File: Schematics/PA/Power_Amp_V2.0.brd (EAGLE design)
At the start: 50.5 x 78.1 mm, 109 parts, among them J1 4_PIN_AMPCONN, J10 OSTVN03A150, J11 OSTVN03A150, J12 OSTVN03A150, J13 OSTVN03A150, J14 OSTVN03A150, J2 1984633, J3 2TERMINAL_SPEAKER, J4 2TERMINAL_SPEAKER, J5 2TERMINAL_SPEAKER, J6 OSTVN03A150, J7 OSTVN03A150, J8 OSTVN03A150, J9 OSTVN03A150, U1 LME49830, U2 LME49830, U3 LME49830

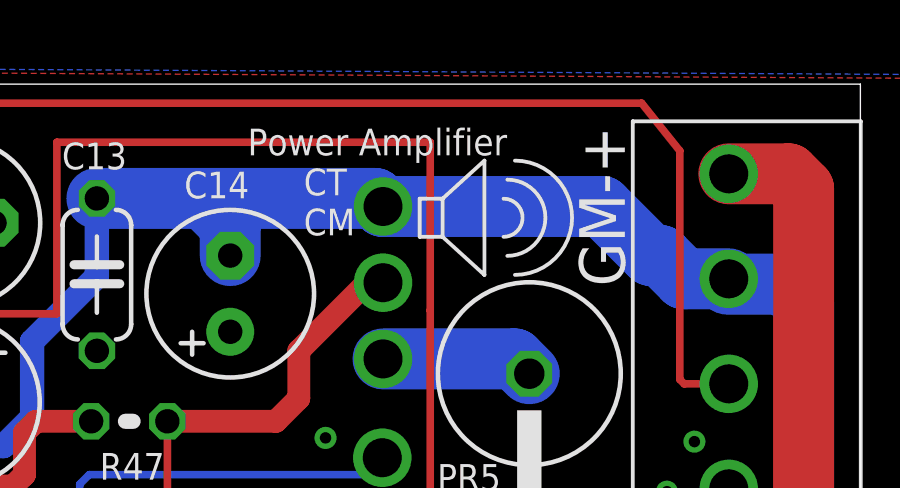
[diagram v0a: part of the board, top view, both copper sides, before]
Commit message: small changes to logo
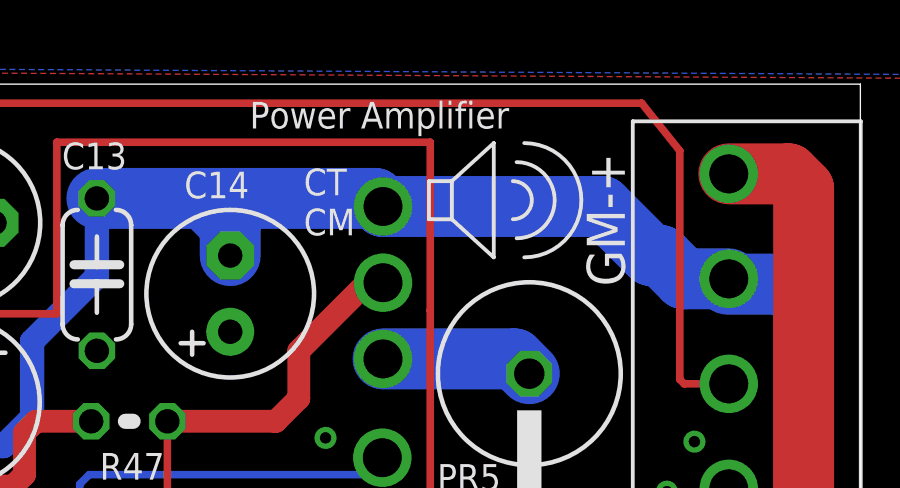
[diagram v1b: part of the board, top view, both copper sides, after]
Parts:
- moved U$48 0.66 mm to (35.6, 74.2)
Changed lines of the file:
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@@
 <grid distance="0.003125" unitdist="mic" unit="inch" style="lines" multiple="1" display="yes" altdistance="0.025" altunitdist="inch" altunit="inch"/>
 <layers>
-<layer number="1" name="Top" color="4" fill="1" visible="no" active="yes"/>
-<layer number="16" name="Bottom" color="1" fill="1" visible="no" active="yes"/>
+<layer number="1" name="Top" color="4" fill="1" visible="yes" active="yes"/>
+<layer number="16" name="Bottom" color="1" fill="1" visible="yes" active="yes"/>
 <layer number="17" name="Pads" color="2" fill="1" visible="yes" active="yes"/>
 <layer number="18" name="Vias" color="2" fill="1" visible="yes" active="yes"/>
@@
 <wire x1="50.47" y1="78.105" x2="1.27" y2="78.105" width="0" layer="20"/>
 <wire x1="0" y1="76.5175" x2="0" y2="0" width="0" layer="20"/>
-<text x="30.043725" y="75.73103125" size="0.889" layer="21" font="vector" ratio="15">Power Amplifier</text>
+<text x="30.112565625" y="76.62565625" size="0.889" layer="21" font="vector" ratio="15">Power Amplifier</text>
 <text x="31.913615625" y="73.064490625" size="0.889" layer="21" font="vector" ratio="15">CT
 CM</text>
@@
 <wire x1="42.874946875" y1="52.071228125" x2="42.874946875" y2="61.11535625" width="2.159" layer="30"/>
 <wire x1="42.874946875" y1="61.11535625" x2="42.997178125" y2="61.20335625" width="2.032" layer="30"/>
-<text x="42.618134375" y="71.365584375" size="1.524" layer="21" rot="R90">GM-+</text>
+<text x="42.618134375" y="71.365584375" size="1.27" layer="21" rot="R90">GM-+</text>
 <text x="42.734415625" y="4.807346875" size="1.778" layer="21" rot="R90">L</text>
 <text x="39.945378125" y="26.134459375" size="1.778" layer="21" rot="R90">B</text>
@@
 </element>
 <element name="U$17" library="PersonalLogos" package="MUSHROOM" value="" x="11.737865625" y="76.558996875" rot="R180"/>
-<element name="U$48" library="PersonalLogos" package="SPEAKER" value="" x="35.271303125" y="73.650784375"/>
+<element name="U$48" library="PersonalLogos" package="SPEAKER" value="" x="35.581084375" y="74.23573125"/>
 <element name="J6" library="Amplifier_Parts" package="OSTVN03A150" value="OSTVN03A150" x="37.753165625" y="50.79018125" rot="R90"/>
 <element name="J7" library="Amplifier_Parts" package="OSTVN03A150" value="OSTVN03A150" x="37.7327625" y="59.07185625" rot="R90"/>
